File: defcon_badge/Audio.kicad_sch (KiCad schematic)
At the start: 16 parts, among them J20 SJ1-3523N, U20 TM8211, U21 TDA1308

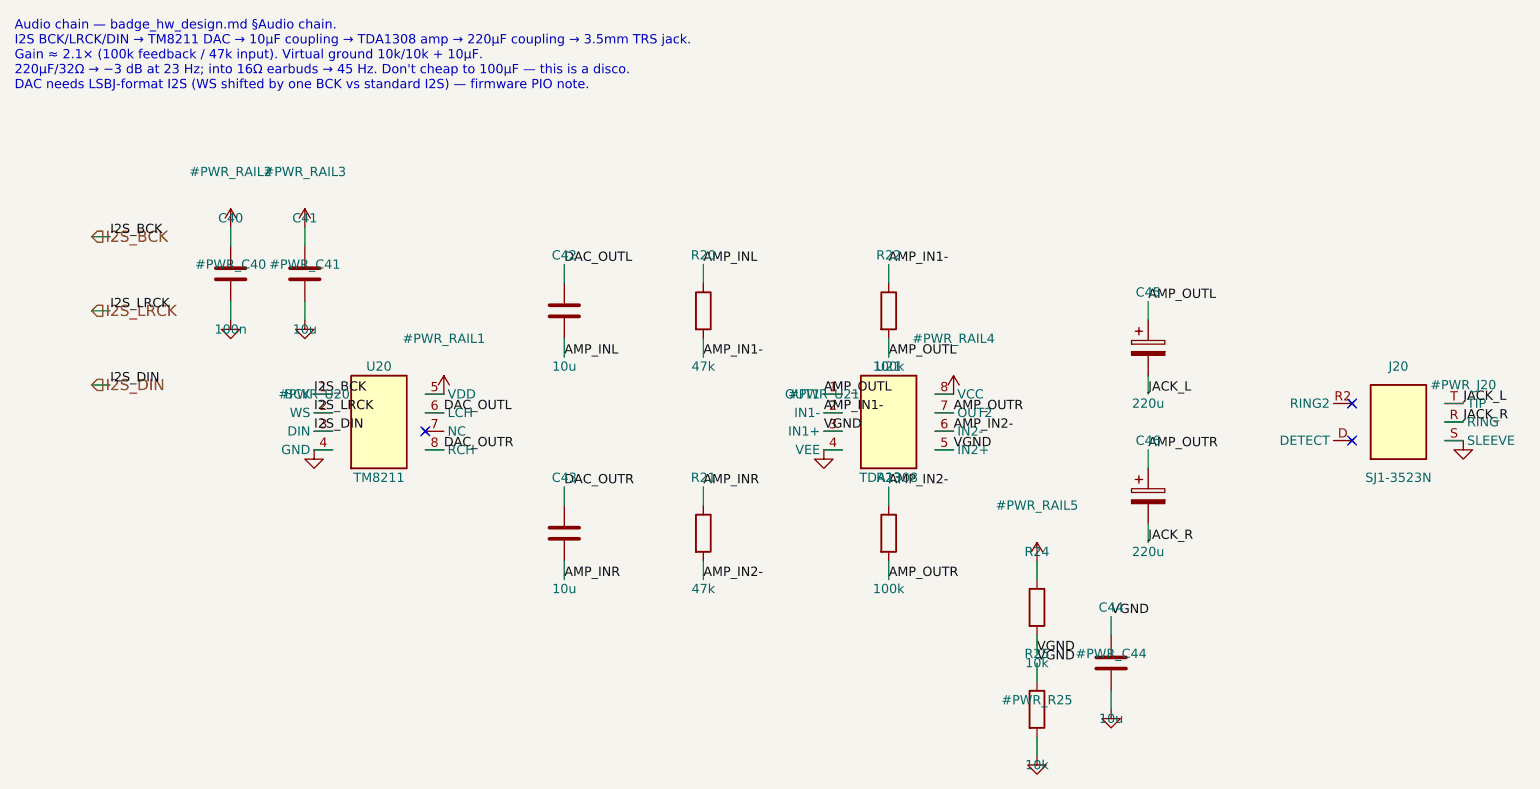
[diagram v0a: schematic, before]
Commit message: Routing redo
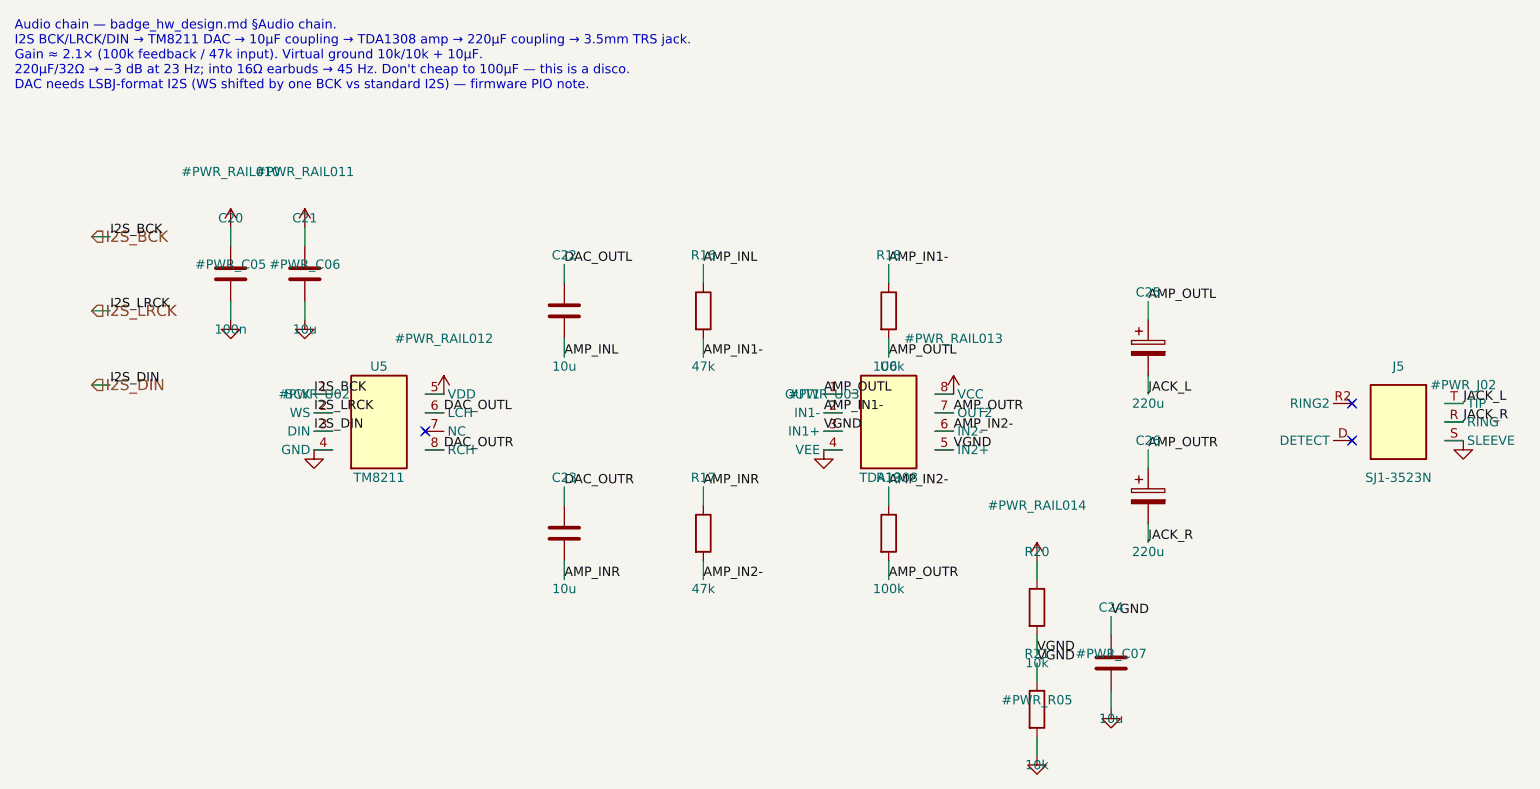
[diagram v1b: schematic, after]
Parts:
- renumbered C40 to C20, C41 to C21, C42 to C22, C43 to C23, C44 to C24, C45 to C25, C46 to C26, J20 to J5, R20 to R16, R21 to R17, R22 to R18, R23 to R19, R24 to R20, R25 to R21, U20 to U5, U21 to U6
